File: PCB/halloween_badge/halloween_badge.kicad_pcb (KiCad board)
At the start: 2 copper layers, 50 x 50 mm, 19 parts, among them U1 ATtiny48-A

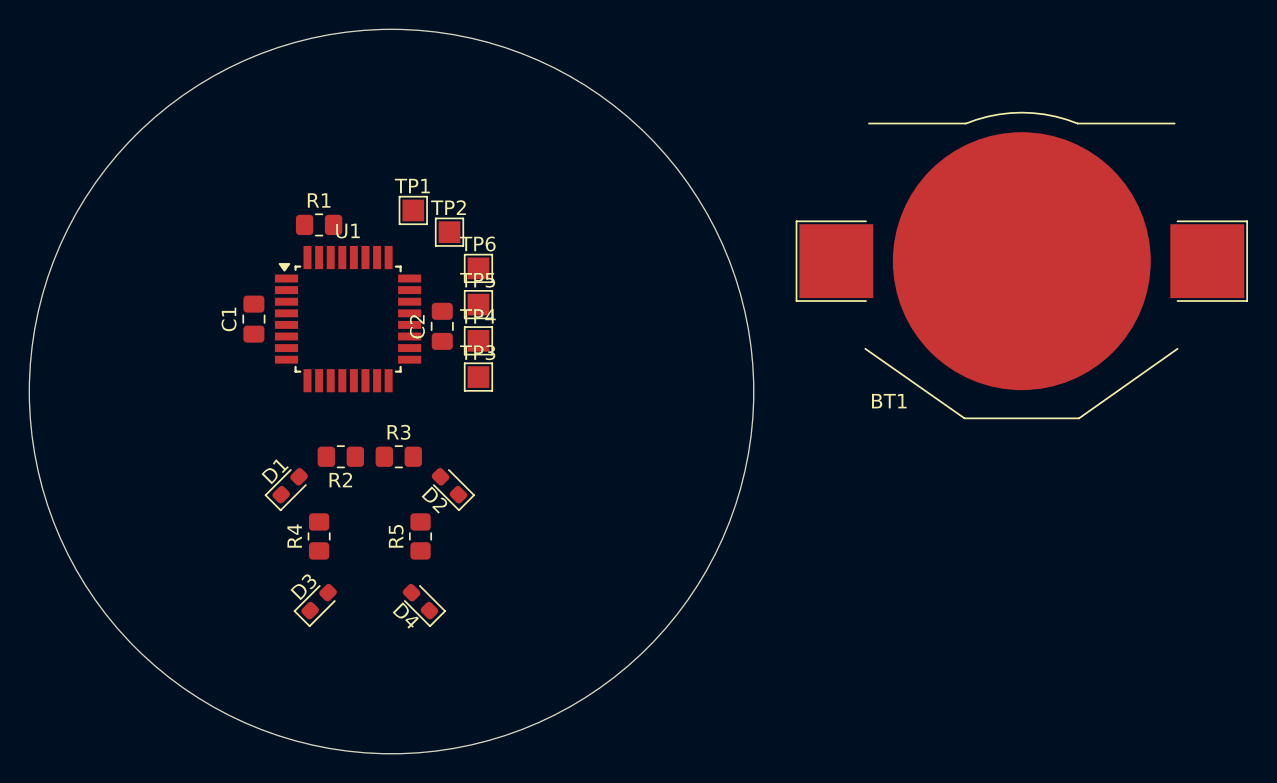
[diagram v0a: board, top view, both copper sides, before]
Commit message: first finished PCB design
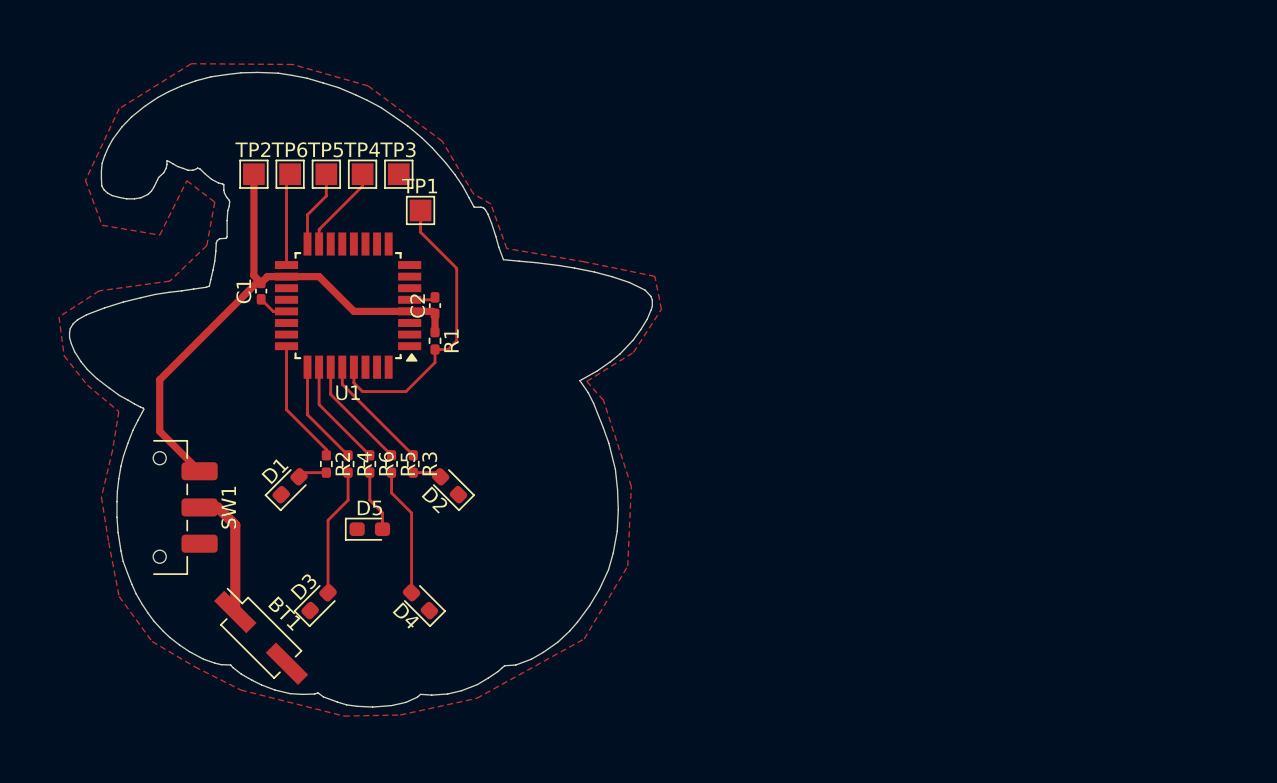
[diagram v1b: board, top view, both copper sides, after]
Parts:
- added D5: LED_Filled, LED_SMD:LED_0603_1608Metric_Pad1.05x0.95mm_HandSolder, F.Cu at (148.5, 109.5)
- added R6: R, Resistor_SMD:R_0402_1005Metric_Pad0.72x0.64mm_HandSolder, F.Cu at (148.5, 105.0)
- added SW1: SW_SPDT, Button_Switch_SMD:SW_SPDT_CK_JS102011SAQN, F.Cu at (134.0, 108.0)
- BT1: footprint Battery:BatteryHolder_Keystone_3002_1x2032 -> Connector_PinHeader_2.54mm:PinHeader_2x01_P2.54mm_Vertical_SMD
- C1, C2: footprint Capacitor_SMD:C_0805_2012Metric_Pad1.18x1.45mm_HandSolder -> Capacitor_SMD:C_0402_1005Metric_Pad0.74x0.62mm_HandSolder
- R1, R2, R3, R4, R5: footprint Resistor_SMD:R_0805_2012Metric_Pad1.20x1.40mm_HandSolder -> Resistor_SMD:R_0402_1005Metric_Pad0.72x0.64mm_HandSolder
- moved BT1 58.6 mm to (141.0, 117.0), turned to -45 degrees
- moved TP3 15.0 mm to (150.5, 85.0)
- moved TP6 14.5 mm to (143.0, 85.0)
- moved TP2 14.1 mm to (140.5, 85.0)
- moved TP4 14.0 mm to (148.0, 85.0)
- moved TP5 13.8 mm to (145.5, 85.0)
- moved R1 11.3 mm to (153.0, 96.5), turned to -90 degrees
- moved R4 5.39 mm to (147.0, 105.0), turned to -90 degrees
- moved R5 5.39 mm to (150.0, 105.0), turned to -90 degrees
- moved C1 2.00 mm to (141.0, 93.1)
- moved C2 1.52 mm to (153.0, 94.1)
- moved R2 1.12 mm to (145.5, 105.0), turned to -90 degrees
- moved R3 1.12 mm to (151.5, 105.0), turned to -90 degrees
- moved U1 0.93 mm to (147.0, 94.1), turned to 180 degrees
- moved TP1 0.50 mm to (152.0, 87.5)
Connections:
- U1 pad 24: unconnected-(U1-PC1-Pad24) -> /led_eye_left
- U1 pad 25: unconnected-(U1-PC2-Pad25) -> /led_mouth_left
- U1 pad 26: unconnected-(U1-PC3-Pad26) -> /led_nose
- U1 pad 27: unconnected-(U1-PC4-Pad27) -> /led_mouth_right
- U1 pad 28: unconnected-(U1-PC5-Pad28) -> /led_eye_right
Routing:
- net +BATT: track 0.00 -> 39.4 mm
- net /nRST: track 0.00 -> 20.4 mm
- net Net-(BT1-+): track 0.00 -> 8.97 mm
- net Net-(D4-A): track 0.00 -> 8.86 mm
- net Net-(D3-A): track 0.00 -> 8.86 mm
- net /led_eye_left: track 0.00 -> 8.67 mm
- net /led_eye_right: track 0.00 -> 8.11 mm
- net /led_mouth_right: track 0.00 -> 7.82 mm
- net /led_nose: track 0.00 -> 7.53 mm
- net /led_mouth_left: track 0.00 -> 7.24 mm
- net /SCK: track 0.00 -> 6.37 mm
- net /MOSI: track 0.00 -> 6.06 mm
- net /MISO: track 0.00 -> 5.36 mm
- net Net-(D5-A): track 0.00 -> 4.26 mm
- net GND: track 0.00 -> 3.91 mm
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- added copper zone on F.Cu, net GND
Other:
- board size 50 x 50 mm -> 40.2 x 43.8 mm
